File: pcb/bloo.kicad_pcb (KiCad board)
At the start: 2 copper layers, 84.9 x 94.9 mm, 107 parts, among them J1 Serial Debug Header, J10 Conn_01x06_Female, J4 Conn_ARM_JTAG_SWD_10, J5 SWD Header, J6 Conn_01x02_Female, J7 Conn_01x02_Female, J8 Conn_01x02_Female, J9 Conn_01x02_Female, M1 M1_Conn, M2 M2_Conn, M3 M1_Conn_Alt, M4 M2_Conn_Alt, Q0 Q_Photo_NPN, Q1 Q_Photo_NPN, Q10 Q_NMOS_GSD, Q11 Q_NMOS_GSD, Q12 Q_NMOS_GSD, Q2 Q_Photo_NPN, Q3 Q_Photo_NPN, Q4 Q_NMOS_SGD, Q5 Q_NMOS_SGD, Q6 Q_NMOS_SGD, Q7 Q_NMOS_SGD, Q8 Q_NMOS_SGD, Q9 Q_NMOS_GSD, SW1 SW, U1 YAAJ_BluePill_SWD_Breakout, U2 L293D, U3 LM1085-5.0, U4 APE8865Y5-33-HF-3

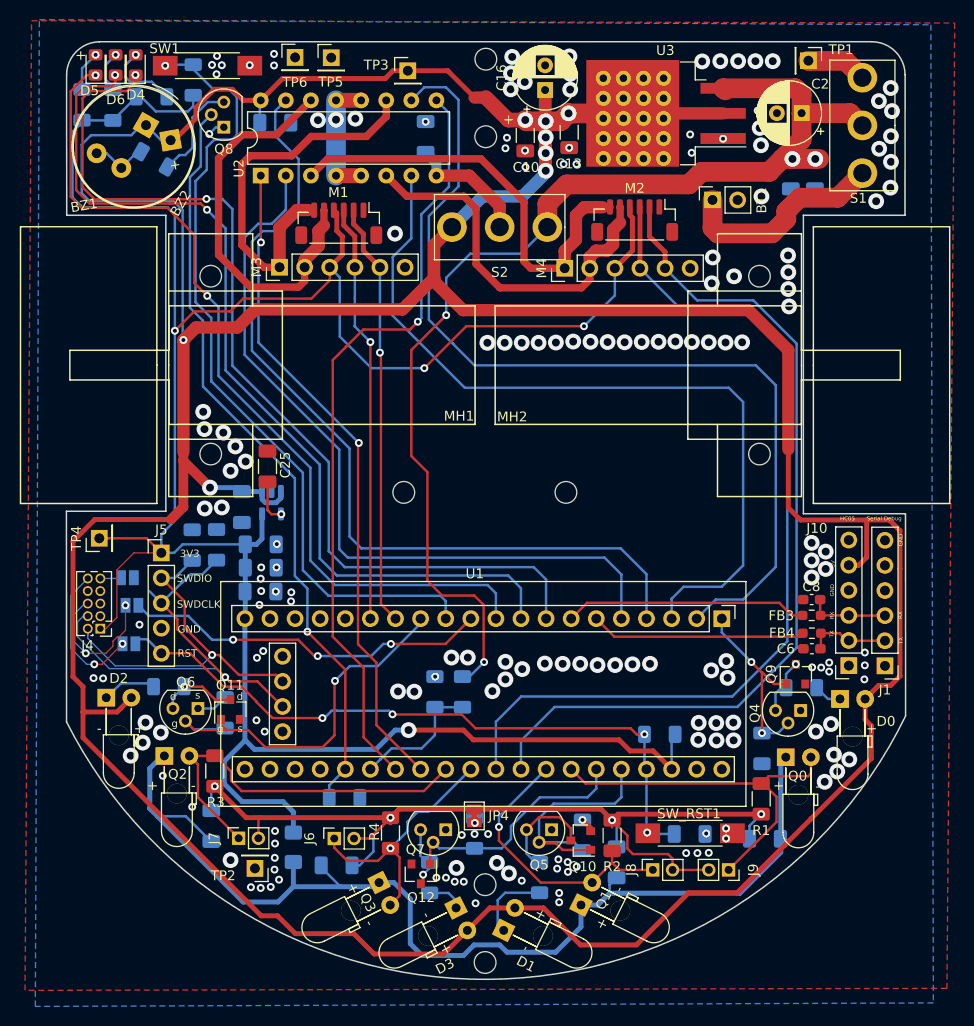
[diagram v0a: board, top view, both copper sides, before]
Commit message: Saved files in KiCAD 7
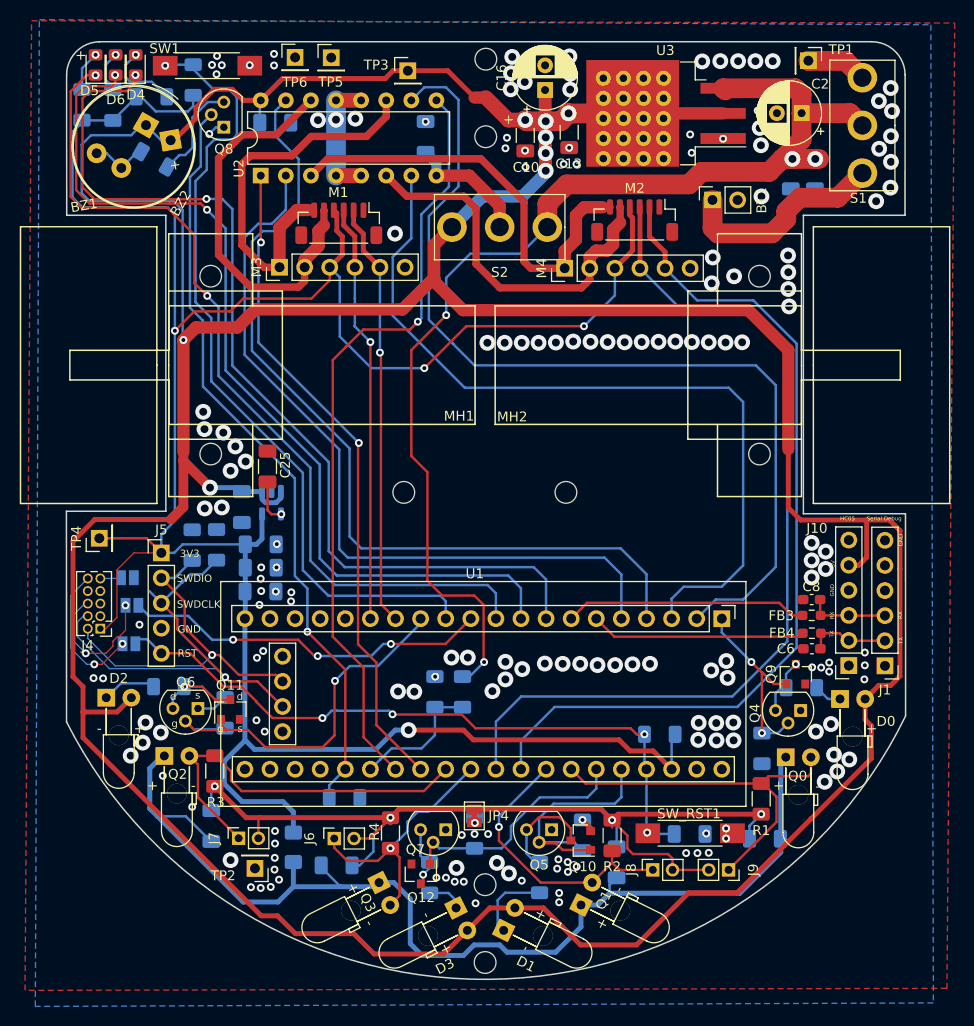
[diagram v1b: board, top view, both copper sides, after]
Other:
- net class Default removed
